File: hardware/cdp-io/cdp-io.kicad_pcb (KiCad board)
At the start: 2 copper layers, 99.1 x 99.1 mm, 33 parts, among them J1 Conn_01x26_Pin, J2 Conn_02x20_Odd_Even, J3 Conn_01x07_Pin, J4 Conn_01x04_Pin, U1 74LS573, U10 74LS175, U2 74LS573, U3 74LS573, U4 74LS573, U5 74LS573, U6 74LS573, U7 74LS14, U8 74LS138, U9 74LS138

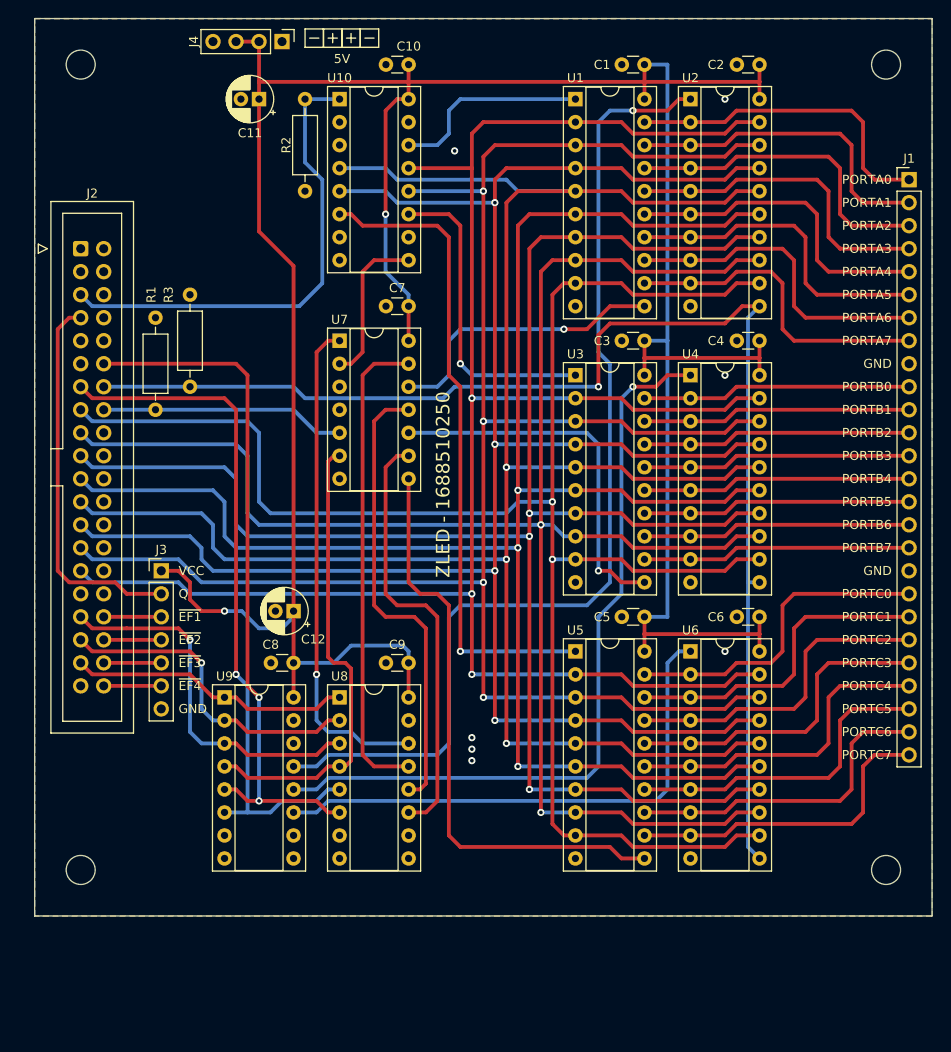
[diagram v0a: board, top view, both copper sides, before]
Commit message: The final version of the IO board. Gerber files added.
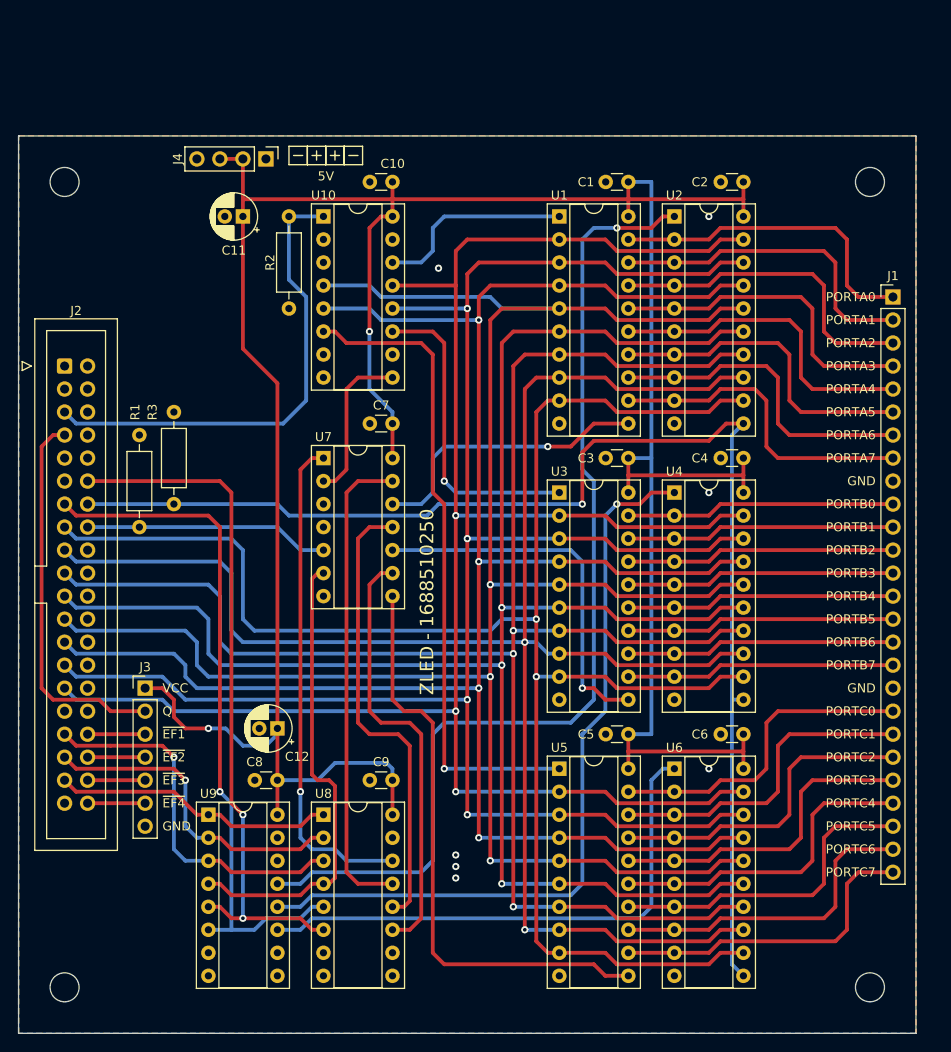
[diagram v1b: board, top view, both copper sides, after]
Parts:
- moved C12 13.1 mm to (128.4, 107.6)
- moved C4 13.1 mm to (179.8, 77.7)
- moved C8 13.1 mm to (128.4, 113.3)
- moved R3 13.1 mm to (117.0, 82.8)
- moved REF** 13.1 mm to (104.9, 136.1)
- moved REF** 13.1 mm to (193.8, 136.1)
- moved U4 13.1 mm to (172.2, 81.5)
- moved C3 13.1 mm to (167.1, 77.7)
- moved C9 13.1 mm to (141.1, 113.3)
- moved U3 13.1 mm to (159.5, 81.5)
- moved U7 13.1 mm to (133.5, 77.7)
- moved C2 13.1 mm to (179.8, 47.2)
- moved J4 13.1 mm to (127.1, 44.7)
- moved REF** 13.1 mm to (193.8, 47.2)
- moved REF** 13.1 mm to (104.9, 47.2)
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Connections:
- U7 pad 3: unconnected-(U7-Pad3) -> GND
